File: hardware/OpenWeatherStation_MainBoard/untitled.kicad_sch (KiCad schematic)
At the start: 1 part, among them J1 RJ45_LED_Shielded

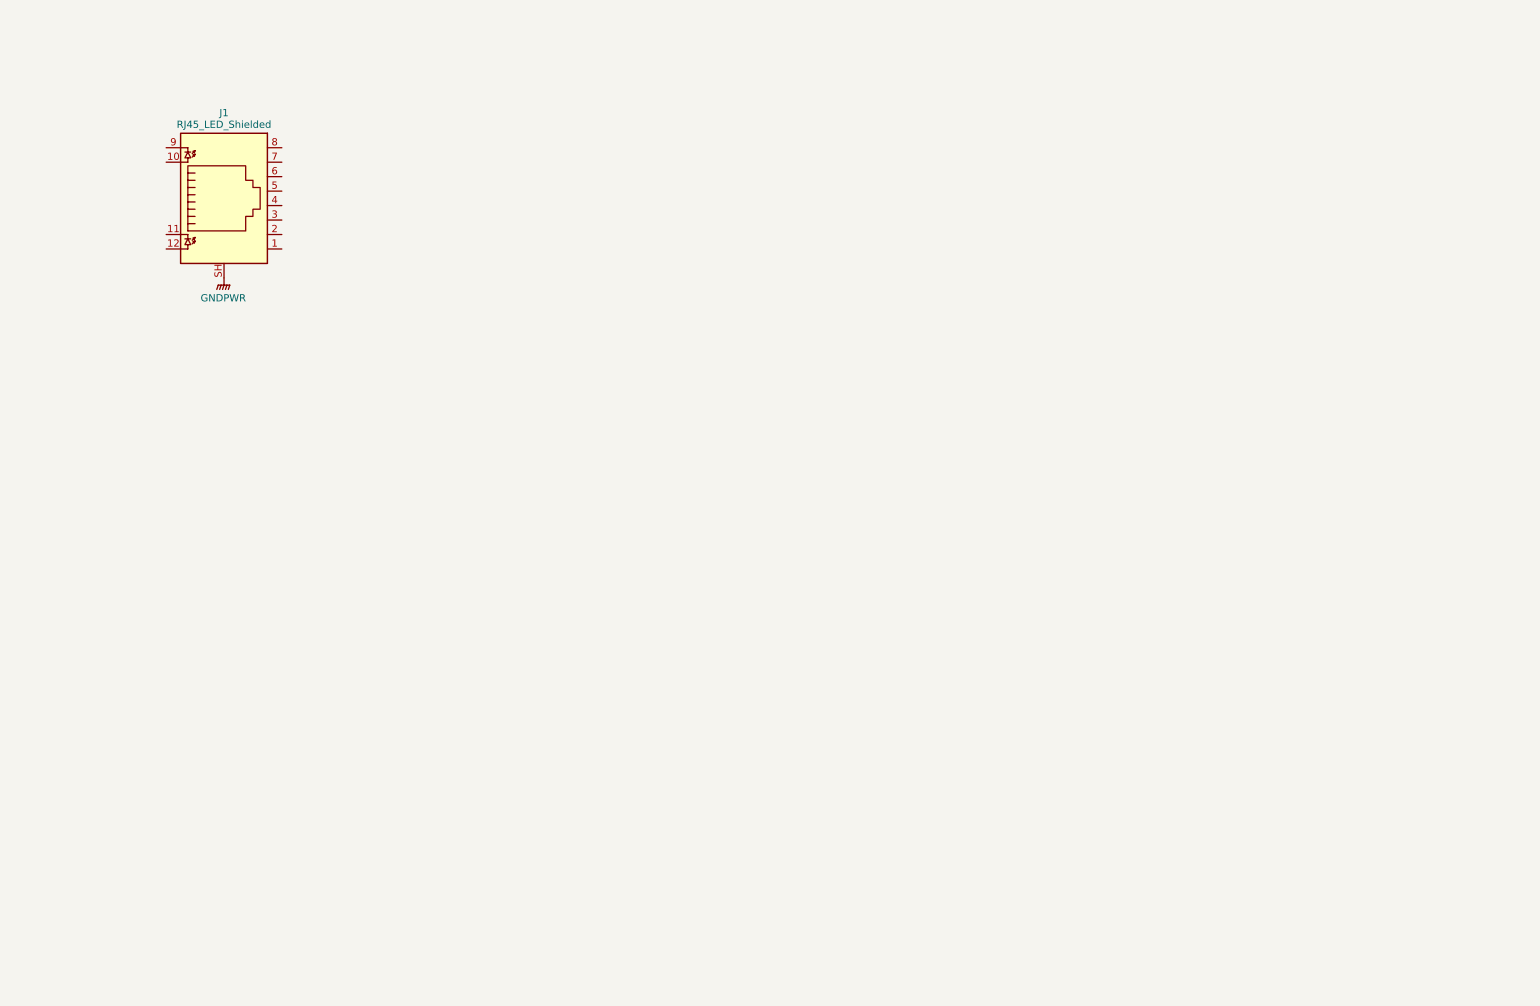
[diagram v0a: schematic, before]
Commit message: poe design wip
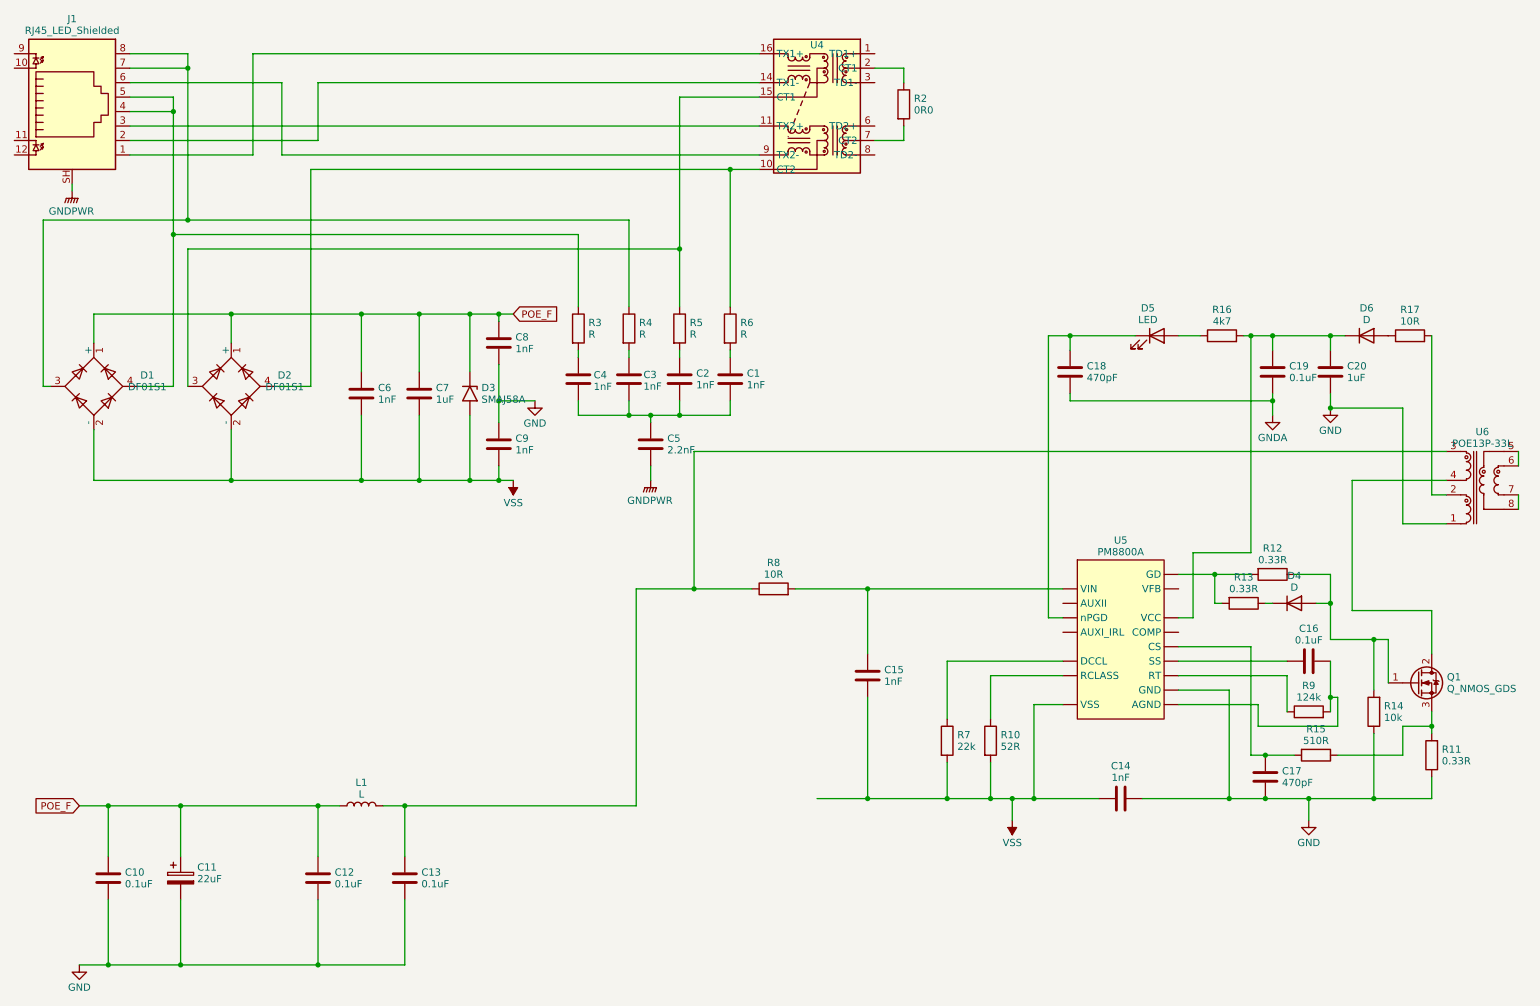
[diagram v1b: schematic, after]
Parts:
- added C1, C14, C15, C2, C3, C4, C6, C8, C9: 1nF, symbol Device:C
- added C10, C12, C13, C16, C19: 0.1uF, symbol Device:C
- added C11: 22uF, symbol Device:C_Polarized
- added C17, C18: 470pF, symbol Device:C
- added C20, C7: 1uF, symbol Device:C
- added C5: 2.2nF, symbol Device:C
- added D1, D2: DF01S1, Diode_SMD:Diode_Bridge_OnSemi_SDIP-4L, symbol Diode_Bridge:DF01S1
- added D3: SMAJ58A, Diode_SMD:D_SMA, symbol Diode:SMAJ58A
- added D4, D6: D, symbol Device:D
- added D5: LED, symbol Device:LED
- added L1: L, symbol Device:L
- added Q1: Q_NMOS_GDS, symbol Device:Q_NMOS_GDS
- added R10: 52R, symbol Device:R
- added R11, R12, R13: 0.33R, symbol Device:R
- added R14: 10k, symbol Device:R
- added R15: 510R, symbol Device:R
- added R16: 4k7, symbol Device:R
- added R17, R8: 10R, symbol Device:R
- added R2: 0R0, symbol Device:R
- added R3, R4, R5, R6: R, symbol Device:R
- added R7: 22k, symbol Device:R
- added R9: 124k, symbol Device:R
- added U4: ~, symbol New_Library:SM13126PEL
- added U5: PM8800A, symbol New_Library:PM8800A
- added U6: POE13P-33L, symbol New_Library:POE13P-33L
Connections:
- net GNDPWR: now also C5.2
- net at J1.1: now also U4.16 (TX1+)
- net at J1.2: now also U4.14 (TX1-)
- net at J1.3: now also U4.11 (TX2+)
- net at J1.4: now also J1.5, D1.4, R3.1
- net at J1.6: now also U4.9 (TX2-)
- net at J1.7: now also J1.8, D1.3, R4.1
- new net: R9.1, U5. (nPGD)
- new net: C16.1, R9.2, U5. (nPGD)
- new net: D2.3, R5.1, U4.15 (CT1)
- new net: C2.1, R5.2
- new net: C3.1, R4.2
- new net: C19.1, C20.1, D6.1 (K), R16.2, U5. (nPGD)
- new net: D4.2 (A), Q1.1 (G), R12.1, R14.2
- new net: C13.1, L1.2, R8.1, U6.3
- new net: C15.2, R8.2, U5. (nPGD)
- new net: Q1.3 (S), R11.2, R15.1
- new net: C17.1, R15.2, U5. (nPGD)
- new net: Q1.2 (D), U6.4
- new net: R17.2, U6.2
- new net: U6.5, U6.6
- new net: U6.7, U6.8
- new net: R2.1, U4.2 (CT1)
- new net: R2.2, U4.7 (CT2)
- new net: R10.1, U5. (nPGD)
- new net: D4.1 (K), R13.1
- new net: R12.2, R13.2, U5. (nPGD)
- new net: C1.2, C2.2, C3.2, C4.2, C5.1
- new net: C4.1, R3.2
- new net: C16.2, U5. (nPGD)
- new net: D2.4, R6.1, U4.10 (CT2)
- new net: D6.2 (A), R17.1
- new net: C18.1, D5.1 (K), U5. (nPGD)
- new net: R7.1, U5. (nPGD)
- new net: C1.1, R6.2
- new net: D5.2 (A), R16.1
- new net GND: C10.2, C11.2, C12.2, C13.2, C14.2, C17.2, C20.2, C8.2, C9.1, R11.1, R14.1, U5. (nPGD), U6.1
- new net GNDA: C18.2, C19.2
- new net POE_F: C10.1, C11.1, C12.1, C6.1, C7.1, C8.1, D1.1 (+), D2.1 (+), D3.1 (A1), L1.1
- new net VSS: C14.1, C15.1, C6.2, C7.2, C9.2, D1.2 (-), D2.2 (-), D3.2 (A2), R10.2, R7.2, U5. (nPGD)
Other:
- moved on the sheet: J1
